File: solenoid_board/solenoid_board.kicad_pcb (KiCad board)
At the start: 2 copper layers, 152.4 x 64.8 mm, 207 parts, among them J1 output, J10 output, J11 output, J12 PORT, J13 PORT, J14 PORT, J15 PORT, J16 PORT, J17 PORT, J18 PORT, J19 PORT, J2 Conn_02x13_Odd_Even, J20 5V in, J21 XT60-M, J3 output, J4 output, J5 output, J6 output, J7 output, J8 output, J9 output, Q1 AOD4184A, Q10 AOD4184A, Q2 AOD4184A, Q3 AOD4184A, Q4 AOD4184A, Q5 AOD4184A, Q6 AOD4184A, Q7 AOD4184A, Q8 AOD4184A, Q9 AOD4184A, SW1 SW_Push, SW10 SW_Push, SW2 SW_Push, SW3 SW_Push, SW4 SW_Push, SW5 SW_Push, SW6 SW_Push, SW7 SW_Push, SW8 SW_Push, SW9 SW_Push, U1 EL357N, U10 EL357N, U11 EL357N, U12 EL357N, U13 EL357N, U14 EL357N, U15 EL357N, U16 EL357N, U17 EL357N, U18 EL357N, U2 EL357N, U3 EL357N, U4 EL357N, U5 EL357N, U6 EL357N, U7 EL357N, U8 EL357N, U9 EL357N

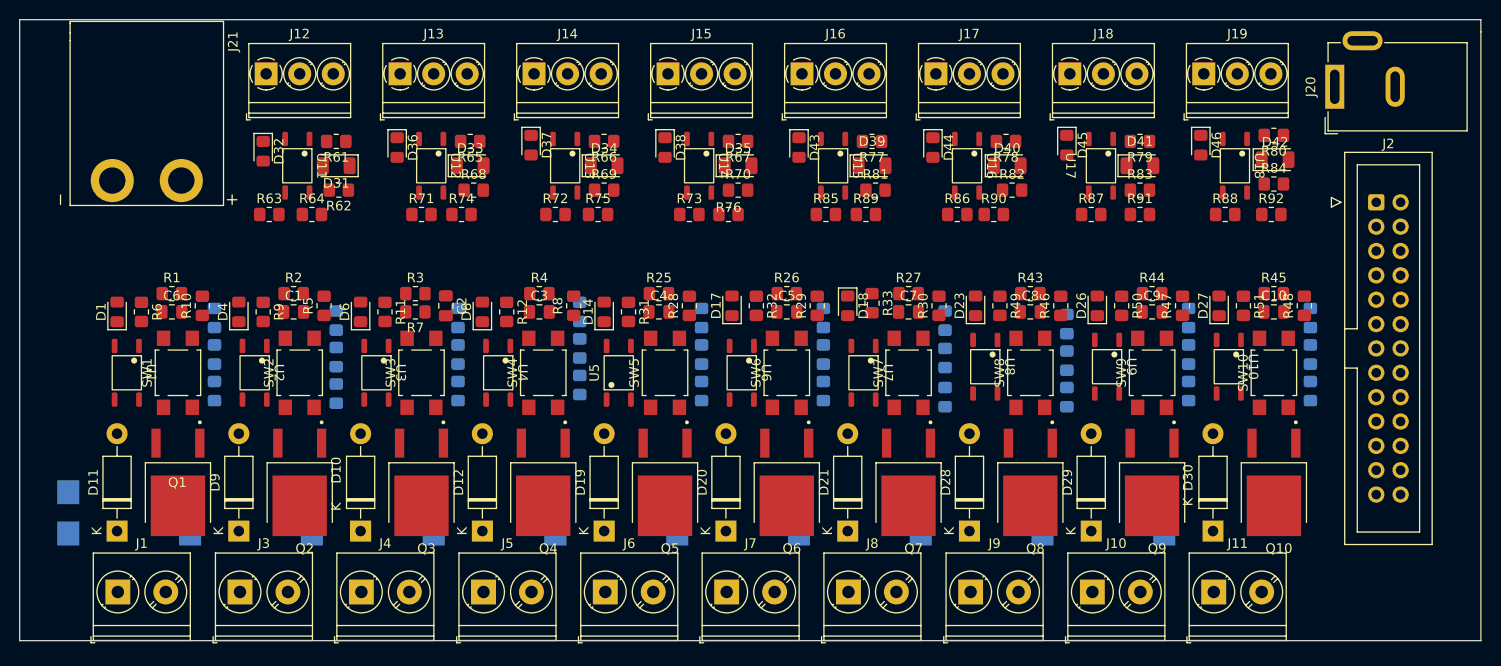
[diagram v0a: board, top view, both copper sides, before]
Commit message: test
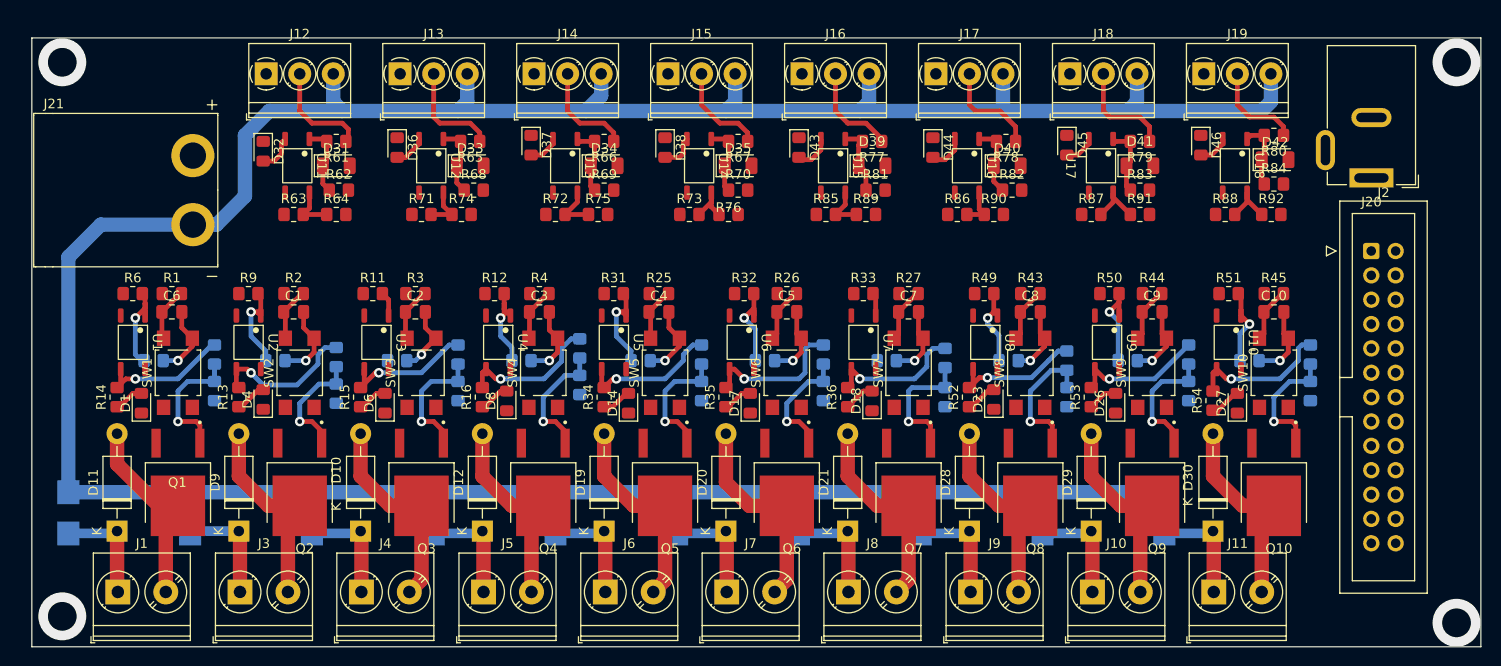
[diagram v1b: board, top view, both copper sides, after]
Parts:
- R10, R28, R29, R30, R46, R47, R48, R5, R7, R8: moved to B.Cu
- R13, R14, R15, R16, R34, R35, R36, R52, R53, R54: moved to F.Cu
- moved R16 13.5 mm to (156.2, 78.7), turned to 90 degrees
- moved R54 13.3 mm to (232.4, 79.1), turned to 90 degrees
- moved R14 13.1 mm to (118.1, 78.7), turned to 90 degrees
- moved R15 13.1 mm to (143.5, 78.7), turned to 90 degrees
- moved R34 13.1 mm to (168.9, 78.7), turned to 90 degrees
- moved R35 13.1 mm to (181.6, 78.7), turned to 90 degrees
- moved R53 13.1 mm to (219.7, 78.7), turned to 90 degrees
- moved R13 12.9 mm to (130.8, 78.7), turned to 90 degrees
- moved R36 12.9 mm to (194.3, 78.7), turned to 90 degrees
- moved R52 12.7 mm to (207.0, 78.7)
- moved D17 10.3 mm to (184.2, 79.4)
- moved D26 10.3 mm to (222.2, 79.4)
- moved D27 10.3 mm to (234.9, 79.4)
- moved J20 10.3 mm to (248.9, 55.9), turned to 180 degrees
- moved D18 10.2 mm to (196.8, 79.1), turned to 90 degrees
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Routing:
- net +24V: track 0.00 -> 307.5 mm
- net Net-(D20-Pad2): track 0.00 -> 22.0 mm
- net Net-(D10-Pad2): track 0.00 -> 21.6 mm
- net Net-(D21-Pad2): track 0.00 -> 21.6 mm
- net Net-(D30-Pad2): track 0.00 -> 21.6 mm
- net Net-(D28-Pad2): track 0.00 -> 21.6 mm
- net Net-(D9-Pad2): track 0.00 -> 21.6 mm
- net Net-(D29-Pad2): track 0.00 -> 21.6 mm
- net Net-(D12-Pad2): track 0.00 -> 21.6 mm
- net Net-(D19-Pad2): track 0.00 -> 21.6 mm
- net Net-(D11-Pad2): track 0.00 -> 20.8 mm
- net Net-(R13-Pad2): track 0.00 -> 15.3 mm, vias 0 -> 1
- net Net-(R35-Pad2): track 0.00 -> 15.2 mm, vias 0 -> 1
- net Net-(R54-Pad2): track 0.00 -> 14.9 mm, vias 0 -> 1
- net Net-(R16-Pad2): track 0.00 -> 14.8 mm, vias 0 -> 1
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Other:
- board size 152.4 x 64.8 mm -> 151.1 x 63.5 mm
